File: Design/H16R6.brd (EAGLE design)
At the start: 30 x 34.6 mm, 113 parts, among them IC1 74LVC2T45HK3-7, P1 HEXABIT_17.32, U1 STM32G0B1CEU6N, X1 XTALL_CSTCE8M00G52

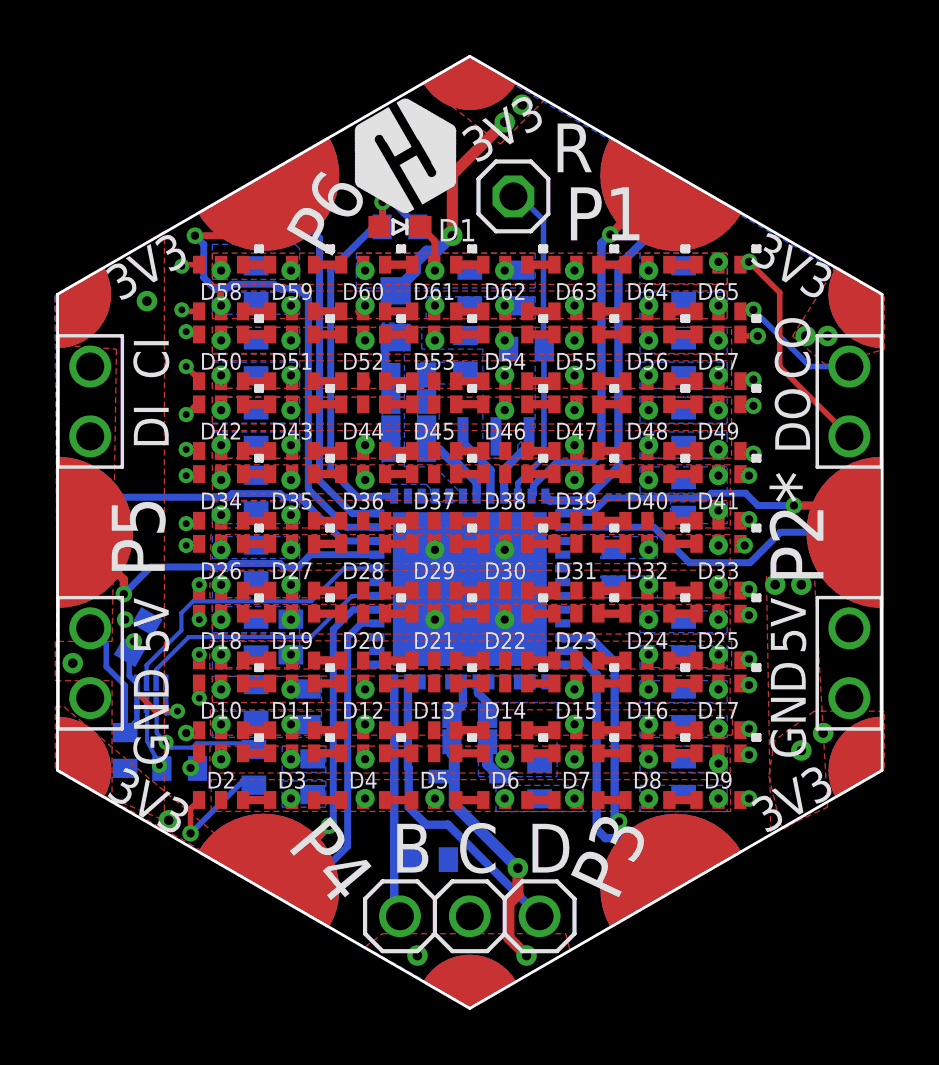
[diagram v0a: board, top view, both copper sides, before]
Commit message: no message
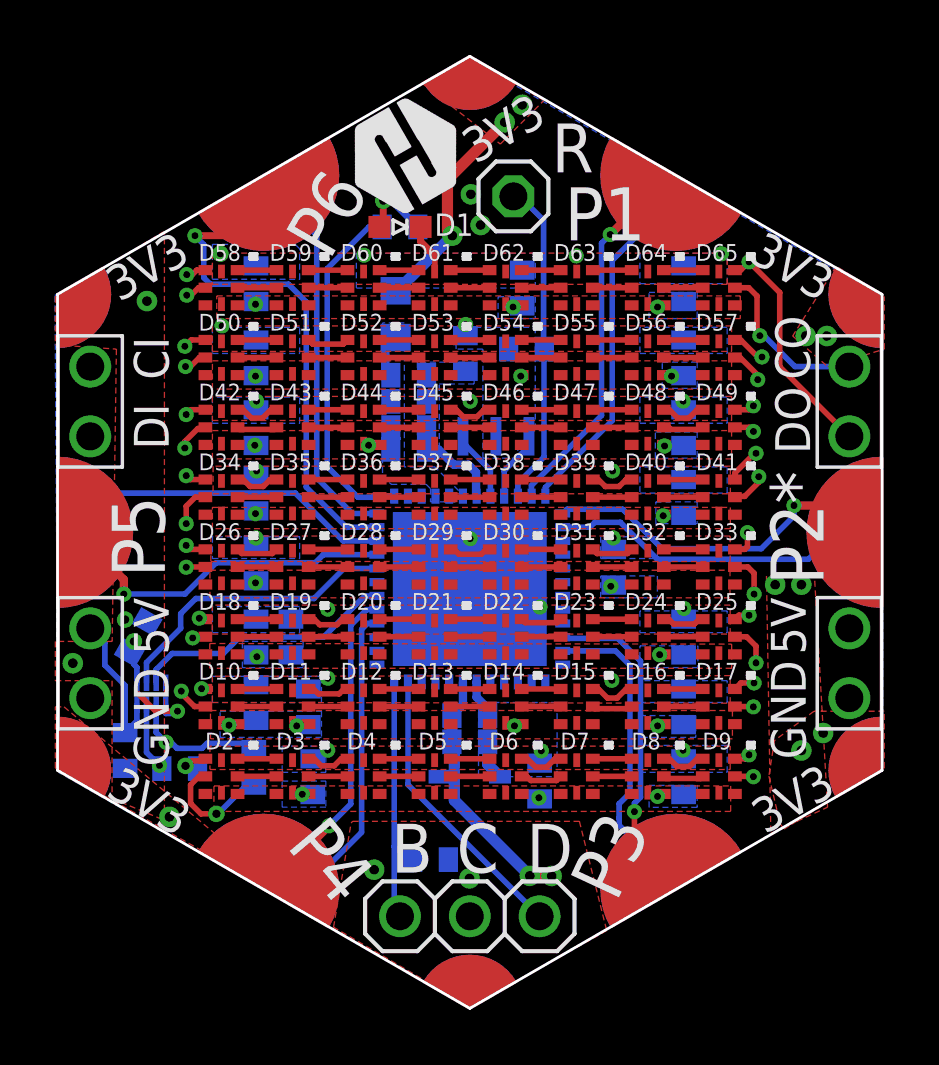
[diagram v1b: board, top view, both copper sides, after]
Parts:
- removed C1: 100nF, HEXABITZ_RCLS:C-0402
- moved SERIAL_IN 27.6 mm to (-13.8, 23.3)
- moved SERIAL_OUT 27.6 mm to (13.8, 23.3)
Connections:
- net +VS: now also D10.VDD1, D11.VDD1, D12.VDD1, D13.VDD1, D14.VDD1, D15.VDD1, D16.VDD1, D17.VDD1, D18.VDD1, D19.VDD1, D2.VDD1, D20.VDD1, D21.VDD1, D22.VDD1, D23.VDD1, D24.VDD1, D25.VDD1, D26.VDD1, D27.VDD1, D28.VDD1, D29.VDD1, D3.VDD1, D30.VDD1, D31.VDD1, D32.VDD1, D33.VDD1, D34.VDD1, D35.VDD1, D36.VDD1, D37.VDD1, D38.VDD1, D39.VDD1, D4.VDD1, D40.VDD1, D41.VDD1, D42.VDD1, D43.VDD1, D44.VDD1, D45.VDD1, D46.VDD1, D47.VDD1, D48.VDD1, D49.VDD1, D5.VDD1, D50.VDD1, D51.VDD1, D52.VDD1, D53.VDD1, D54.VDD1, D55.VDD1, D56.VDD1, D57.VDD1, D58.VDD1, D59.VDD1, D6.VDD1, D60.VDD1, D61.VDD1, D62.VDD1, D63.VDD1, D64.VDD1, D65.VDD1, D7.VDD1, D8.VDD1, D9.VDD1; no longer C1.1
- net CKI: now also SERIAL_IN.1; no longer SERIAL_OUT.1
- net CKO: now also D65.CO, SERIAL_OUT.1; no longer D65.CKO, SERIAL_IN.1
- net GND: no longer C1.2
- net L1_CLK: now also D10.CI, D9.CO; no longer D10.CKI, D9.CKO
- net L1_DATA: now also D10.DI, D9.DO; no longer D10.SDI, D9.SDO
- net L2_CLK: now also D17.CO, D18.CI; no longer D17.CKO, D18.CKI
- net L2_DATA: now also D17.DO, D18.DI; no longer D17.SDO, D18.SDI
- net L3_CLK: now also D25.CO, D26.CI; no longer D25.CKO, D26.CKI
- net L3_DATA: now also D25.DO, D26.DI; no longer D25.SDO, D26.SDI
- net L4_CLK: now also D33.CO, D34.CI; no longer D33.CKO, D34.CKI
- net L4_DATA: now also D33.DO, D34.DI; no longer D33.SDO, D34.SDI
- net L5_CLK: now also D41.CO, D42.CI; no longer D41.CKO, D42.CKI
- net L5_DATA: now also D41.DO, D42.DI; no longer D41.SDO, D42.SDI
- net L6_CLK: now also D49.CO, D50.CI; no longer D49.CKO, D50.CKI
- net L6_DATA: now also D49.DO, D50.DI; no longer D49.SDO, D50.SDI
- net L7_CLK: now also D57.CO, D58.CI; no longer D57.CKO, D58.CKI
- net L7_DATA: now also D57.DO, D58.DI; no longer D57.SDO, D58.SDI
- net N$1: now also D3.DO, D4.DI; no longer D3.SDO, D4.SDI
- net N$10: now also D8.CO, D9.CI; no longer D8.CKO, D9.CKI
- net N$100: now also D45.DO, D46.DI; no longer D45.SDO, D46.SDI
- net N$101: now also D45.CO, D46.CI; no longer D45.CKO, D46.CKI
- net N$102: now also D46.CO, D47.CI; no longer D46.CKO, D47.CKI
- net N$103: now also D46.DO, D47.DI; no longer D46.SDO, D47.SDI
- net N$104: now also D47.CO, D48.CI; no longer D47.CKO, D48.CKI
- net N$105: now also D47.DO, D48.DI; no longer D47.SDO, D48.SDI
- net N$106: now also D12.DO, D13.DI; no longer D12.SDO, D13.SDI
- net N$107: now also D13.DO, D14.DI; no longer D13.SDO, D14.SDI
- net N$108: now also D13.CO, D14.CI; no longer D13.CKO, D14.CKI
- net N$109: now also D14.CO, D15.CI; no longer D14.CKO, D15.CKI
- net N$11: now also D7.CO, D8.CI; no longer D7.CKO, D8.CKI
- net N$110: now also D14.DO, D15.DI; no longer D14.SDO, D15.SDI
- net N$111: now also D15.CO, D16.CI; no longer D15.CKO, D16.CKI
- net N$112: now also D15.DO, D16.DI; no longer D15.SDO, D16.SDI
- net N$113: now also D4.CO, D5.CI; no longer D4.CKO, D5.CKI
- net N$114: now also D4.DO, D5.DI; no longer D4.SDO, D5.SDI
- net N$115: now also D6.CO, D7.CI; no longer D6.CKO, D7.CKI
- net N$116: now also D6.DO, D7.DI; no longer D6.SDO, D7.SDI
- net N$119: now also D2.DI; no longer D2.SDI
- net N$12: now also D7.DO, D8.DI; no longer D7.SDO, D8.SDI
- net N$120: now also D2.CI; no longer D2.CKI
- net N$13: now also D5.CO, D6.CI; no longer D5.CKO, D6.CKI
- net N$14: now also D5.DO, D6.DI; no longer D5.SDO, D6.SDI
- net N$15: now also D16.CO, D17.CI; no longer D16.CKO, D17.CKI
- net N$16: now also D16.DO, D17.DI; no longer D16.SDO, D17.SDI
- net N$17: now also D10.CO, D11.CI; no longer D10.CKO, D11.CKI
- net N$18: now also D10.DO, D11.DI; no longer D10.SDO, D11.SDI
- net N$19: now also D11.CO, D12.CI; no longer D11.CKO, D12.CKI
- net N$2: now also D3.CO, D4.CI; no longer D3.CKO, D4.CKI
- net N$20: now also D11.DO, D12.DI; no longer D11.SDO, D12.SDI
- net N$21: now also D12.CO, D13.CI; no longer D12.CKO, D13.CKI
- net N$22: now also D18.CO, D19.CI; no longer D18.CKO, D19.CKI
- net N$23: now also D18.DO, D19.DI; no longer D18.SDO, D19.SDI
- net N$24: now also D19.CO, D20.CI; no longer D19.CKO, D20.CKI
- net N$25: now also D19.DO, D20.DI; no longer D19.SDO, D20.SDI
- net N$26: now also D20.CO, D21.CI; no longer D20.CKO, D21.CKI
- net N$27: now also D20.DO, D21.DI; no longer D20.SDO, D21.SDI
- net N$28: now also D21.CO, D22.CI; no longer D21.CKO, D22.CKI
- net N$29: now also D21.DO, D22.DI; no longer D21.SDO, D22.SDI
- net N$30: now also D22.CO, D23.CI; no longer D22.CKO, D23.CKI
- net N$31: now also D22.DO, D23.DI; no longer D22.SDO, D23.SDI
- net N$32: now also D23.CO, D24.CI; no longer D23.CKO, D24.CKI
- net N$33: now also D23.DO, D24.DI; no longer D23.SDO, D24.SDI
- net N$34: now also D24.CO, D25.CI; no longer D24.CKO, D25.CKI
- net N$35: now also D24.DO, D25.DI; no longer D24.SDO, D25.SDI
- net N$36: now also D26.CO, D27.CI; no longer D26.CKO, D27.CKI
- net N$37: now also D26.DO, D27.DI; no longer D26.SDO, D27.SDI
- net N$38: now also D27.CO, D28.CI; no longer D27.CKO, D28.CKI
- net N$39: now also D27.DO, D28.DI; no longer D27.SDO, D28.SDI
- net N$40: now also D28.CO, D29.CI; no longer D28.CKO, D29.CKI
- net N$41: now also D28.DO, D29.DI; no longer D28.SDO, D29.SDI
- net N$42: now also D29.CO, D30.CI; no longer D29.CKO, D30.CKI
- net N$43: now also D29.DO, D30.DI; no longer D29.SDO, D30.SDI
- net N$44: now also D31.CO, D32.CI; no longer D31.CKO, D32.CKI
- net N$45: now also D31.DO, D32.DI; no longer D31.SDO, D32.SDI
- net N$46: now also D30.CO, D31.CI; no longer D30.CKO, D31.CKI
- net N$47: now also D30.DO, D31.DI; no longer D30.SDO, D31.SDI
- net N$48: now also D32.CO, D33.CI; no longer D32.CKO, D33.CKI
- net N$49: now also D32.DO, D33.DI; no longer D32.SDO, D33.SDI
- net N$50: now also D34.CO, D35.CI; no longer D34.CKO, D35.CKI
- net N$51: now also D34.DO, D35.DI; no longer D34.SDO, D35.SDI
- net N$52: now also D35.CO, D36.CI; no longer D35.CKO, D36.CKI
- net N$53: now also D35.DO, D36.DI; no longer D35.SDO, D36.SDI
- net N$54: now also D36.CO, D37.CI; no longer D36.CKO, D37.CKI
- net N$55: now also D36.DO, D37.DI; no longer D36.SDO, D37.SDI
- net N$56: now also D37.CO, D38.CI; no longer D37.CKO, D38.CKI
- net N$57: now also D37.DO, D38.DI; no longer D37.SDO, D38.SDI
- net N$58: now also D38.CO, D39.CI; no longer D38.CKO, D39.CKI
- net N$59: now also D38.DO, D39.DI; no longer D38.SDO, D39.SDI
- net N$60: now also D40.CO, D41.CI; no longer D40.CKO, D41.CKI
- net N$61: now also D40.DO, D41.DI; no longer D40.SDO, D41.SDI
- net N$62: now also D39.CO, D40.CI; no longer D39.CKO, D40.CKI
- net N$63: now also D39.DO, D40.DI; no longer D39.SDO, D40.SDI
- net N$64: now also D48.CO, D49.CI; no longer D48.CKO, D49.CKI
- net N$65: now also D48.DO, D49.DI; no longer D48.SDO, D49.SDI
- net N$66: now also D56.CO, D57.CI; no longer D56.CKO, D57.CKI
- net N$67: now also D56.DO, D57.DI; no longer D56.SDO, D57.SDI
- net N$68: now also D64.CO, D65.CI; no longer D64.CKO, D65.CKI
- net N$69: now also D64.DO, D65.DI; no longer D64.SDO, D65.SDI
- net N$7: now also D2.DO, D3.DI; no longer D2.SDO, D3.SDI
- net N$70: now also D55.DO, D56.DI; no longer D55.SDO, D56.SDI
- net N$71: now also D55.CO, D56.CI; no longer D55.CKO, D56.CKI
- net N$72: now also D63.CO, D64.CI; no longer D63.CKO, D64.CKI
- net N$73: now also D63.DO, D64.DI; no longer D63.SDO, D64.SDI
- net N$74: now also D54.CO, D55.CI; no longer D54.CKO, D55.CKI
- net N$75: now also D54.DO, D55.DI; no longer D54.SDO, D55.SDI
- net N$76: now also D62.CO, D63.CI; no longer D62.CKO, D63.CKI
- net N$77: now also D62.DO, D63.DI; no longer D62.SDO, D63.SDI
- net N$78: now also D61.DO, D62.DI; no longer D61.SDO, D62.SDI
- net N$79: now also D61.CO, D62.CI; no longer D61.CKO, D62.CKI
- net N$8: now also D2.CO, D3.CI; no longer D2.CKO, D3.CKI
- net N$80: now also D60.CO, D61.CI; no longer D60.CKO, D61.CKI
- net N$81: now also D60.DO, D61.DI; no longer D60.SDO, D61.SDI
- net N$82: now also D59.CO, D60.CI; no longer D59.CKO, D60.CKI
- net N$83: now also D59.DO, D60.DI; no longer D59.SDO, D60.SDI
- net N$84: now also D58.DO, D59.DI; no longer D58.SDO, D59.SDI
- net N$85: now also D58.CO, D59.CI; no longer D58.CKO, D59.CKI
- net N$86: now also D53.DO, D54.DI; no longer D53.SDO, D54.SDI
- net N$87: now also D53.CO, D54.CI; no longer D53.CKO, D54.CKI
- net N$88: now also D51.CO, D52.CI; no longer D51.CKO, D52.CKI
- net N$89: now also D51.DO, D52.DI; no longer D51.SDO, D52.SDI
- net N$9: now also D8.DO, D9.DI; no longer D8.SDO, D9.SDI
- net N$90: now also D52.DO, D53.DI; no longer D52.SDO, D53.SDI
- net N$91: now also D52.CO, D53.CI; no longer D52.CKO, D53.CKI
- net N$92: now also D50.DO, D51.DI; no longer D50.SDO, D51.SDI
- net N$93: now also D50.CO, D51.CI; no longer D50.CKO, D51.CKI
- net N$94: now also D42.CO, D43.CI; no longer D42.CKO, D43.CKI
- net N$95: now also D42.DO, D43.DI; no longer D42.SDO, D43.SDI
- net N$96: now also D43.CO, D44.CI; no longer D43.CKO, D44.CKI
- net N$97: now also D43.DO, D44.DI; no longer D43.SDO, D44.SDI
- net N$98: now also D44.CO, D45.CI; no longer D44.CKO, D45.CKI
- net N$99: now also D44.DO, D45.DI; no longer D44.SDO, D45.SDI
- net SDI: now also SERIAL_IN.2; no longer SERIAL_OUT.2
- net SDO: now also D65.DO, SERIAL_OUT.2; no longer D65.SDO, SERIAL_IN.2
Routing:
- net L3_CLK: track 21.8 -> 24.4 mm
- net VDD: track 24.2 -> 21.9 mm
- net L1_CLK: track 22.5 -> 24.8 mm
- net L4_CLK: track 22.5 -> 24.7 mm
- net +VS: track 9.67 -> 11.8 mm, vias 44 -> 22
- net L5_CLK: track 22.6 -> 24.5 mm
- net L2_CLK: track 21.7 -> 23.0 mm
- net CKO: track 4.84 -> 6.14 mm
- net USART4_RX: track 14.0 -> 12.9 mm
- net USART2_TX: track 11.8 -> 12.9 mm
- net L1_DATA: track 21.7 -> 22.7 mm
- net L4_DATA: track 22.0 -> 23.0 mm
- net USART3_RX: track 10.4 -> 11.3 mm
- net USART3_TX: track 10.7 -> 11.5 mm
- net USART4_TX: track 14.1 -> 13.4 mm
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
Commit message: Replace the led APA-102-2020-6 with APA-102-2020-8
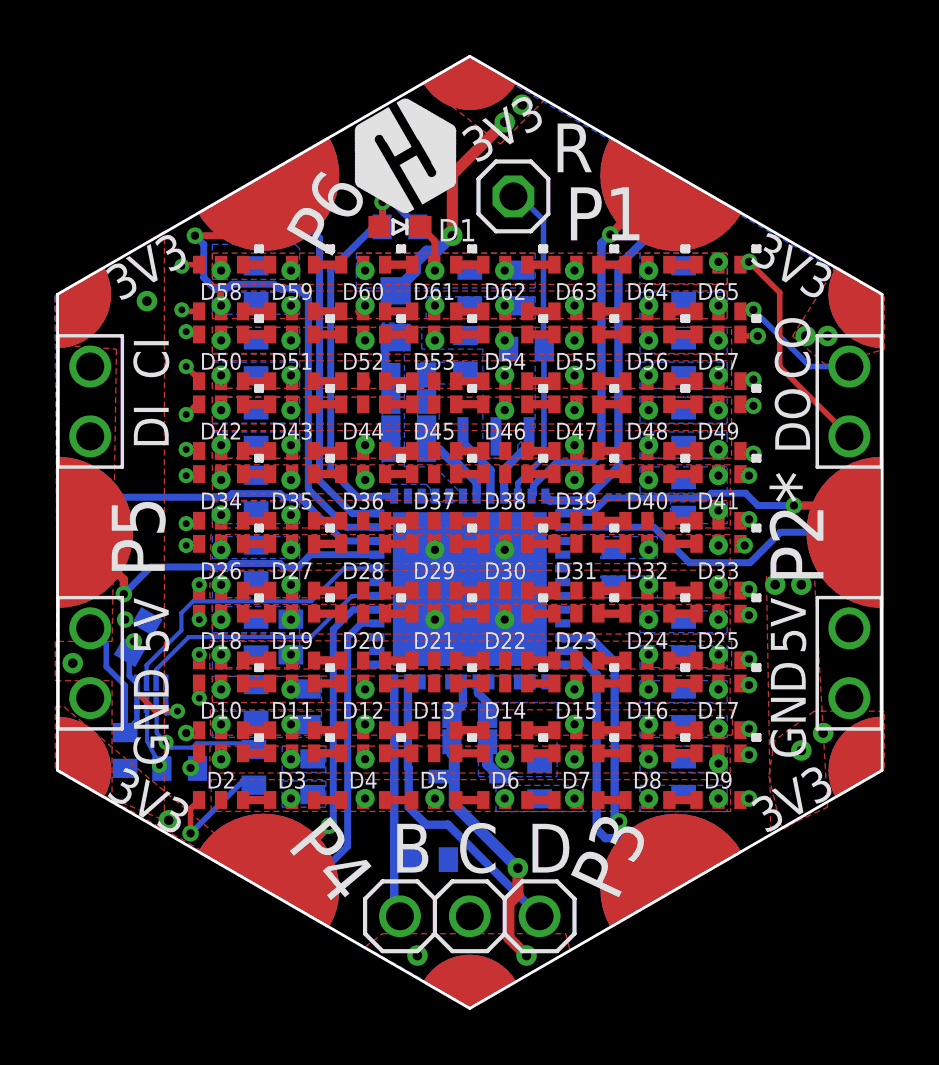
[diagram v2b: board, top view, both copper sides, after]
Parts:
- added C1: 100nF, HEXABITZ_RCLS:C-0402
- moved SERIAL_IN 27.6 mm to (13.8, 23.3)
- moved SERIAL_OUT 27.6 mm to (-13.8, 23.3)
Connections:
- net +VS: now also C1.1; no longer D10.VDD1, D11.VDD1, D12.VDD1, D13.VDD1, D14.VDD1, D15.VDD1, D16.VDD1, D17.VDD1, D18.VDD1, D19.VDD1, D2.VDD1, D20.VDD1, D21.VDD1, D22.VDD1, D23.VDD1, D24.VDD1, D25.VDD1, D26.VDD1, D27.VDD1, D28.VDD1, D29.VDD1, D3.VDD1, D30.VDD1, D31.VDD1, D32.VDD1, D33.VDD1, D34.VDD1, D35.VDD1, D36.VDD1, D37.VDD1, D38.VDD1, D39.VDD1, D4.VDD1, D40.VDD1, D41.VDD1, D42.VDD1, D43.VDD1, D44.VDD1, D45.VDD1, D46.VDD1, D47.VDD1, D48.VDD1, D49.VDD1, D5.VDD1, D50.VDD1, D51.VDD1, D52.VDD1, D53.VDD1, D54.VDD1, D55.VDD1, D56.VDD1, D57.VDD1, D58.VDD1, D59.VDD1, D6.VDD1, D60.VDD1, D61.VDD1, D62.VDD1, D63.VDD1, D64.VDD1, D65.VDD1, D7.VDD1, D8.VDD1, D9.VDD1
- net CKI: now also SERIAL_OUT.1; no longer SERIAL_IN.1
- net CKO: now also D65.CKO, SERIAL_IN.1; no longer D65.CO, SERIAL_OUT.1
- net GND: now also C1.2
- net L1_CLK: now also D10.CKI, D9.CKO; no longer D10.CI, D9.CO
- net L1_DATA: now also D10.SDI, D9.SDO; no longer D10.DI, D9.DO
- net L2_CLK: now also D17.CKO, D18.CKI; no longer D17.CO, D18.CI
- net L2_DATA: now also D17.SDO, D18.SDI; no longer D17.DO, D18.DI
- net L3_CLK: now also D25.CKO, D26.CKI; no longer D25.CO, D26.CI
- net L3_DATA: now also D25.SDO, D26.SDI; no longer D25.DO, D26.DI
- net L4_CLK: now also D33.CKO, D34.CKI; no longer D33.CO, D34.CI
- net L4_DATA: now also D33.SDO, D34.SDI; no longer D33.DO, D34.DI
- net L5_CLK: now also D41.CKO, D42.CKI; no longer D41.CO, D42.CI
- net L5_DATA: now also D41.SDO, D42.SDI; no longer D41.DO, D42.DI
- net L6_CLK: now also D49.CKO, D50.CKI; no longer D49.CO, D50.CI
- net L6_DATA: now also D49.SDO, D50.SDI; no longer D49.DO, D50.DI
- net L7_CLK: now also D57.CKO, D58.CKI; no longer D57.CO, D58.CI
- net L7_DATA: now also D57.SDO, D58.SDI; no longer D57.DO, D58.DI
- net N$1: now also D3.SDO, D4.SDI; no longer D3.DO, D4.DI
- net N$10: now also D8.CKO, D9.CKI; no longer D8.CO, D9.CI
- net N$100: now also D45.SDO, D46.SDI; no longer D45.DO, D46.DI
- net N$101: now also D45.CKO, D46.CKI; no longer D45.CO, D46.CI
- net N$102: now also D46.CKO, D47.CKI; no longer D46.CO, D47.CI
- net N$103: now also D46.SDO, D47.SDI; no longer D46.DO, D47.DI
- net N$104: now also D47.CKO, D48.CKI; no longer D47.CO, D48.CI
- net N$105: now also D47.SDO, D48.SDI; no longer D47.DO, D48.DI
- net N$106: now also D12.SDO, D13.SDI; no longer D12.DO, D13.DI
- net N$107: now also D13.SDO, D14.SDI; no longer D13.DO, D14.DI
- net N$108: now also D13.CKO, D14.CKI; no longer D13.CO, D14.CI
- net N$109: now also D14.CKO, D15.CKI; no longer D14.CO, D15.CI
- net N$11: now also D7.CKO, D8.CKI; no longer D7.CO, D8.CI
- net N$110: now also D14.SDO, D15.SDI; no longer D14.DO, D15.DI
- net N$111: now also D15.CKO, D16.CKI; no longer D15.CO, D16.CI
- net N$112: now also D15.SDO, D16.SDI; no longer D15.DO, D16.DI
- net N$113: now also D4.CKO, D5.CKI; no longer D4.CO, D5.CI
- net N$114: now also D4.SDO, D5.SDI; no longer D4.DO, D5.DI
- net N$115: now also D6.CKO, D7.CKI; no longer D6.CO, D7.CI
- net N$116: now also D6.SDO, D7.SDI; no longer D6.DO, D7.DI
- net N$119: now also D2.SDI; no longer D2.DI
- net N$12: now also D7.SDO, D8.SDI; no longer D7.DO, D8.DI
- net N$120: now also D2.CKI; no longer D2.CI
- net N$13: now also D5.CKO, D6.CKI; no longer D5.CO, D6.CI
- net N$14: now also D5.SDO, D6.SDI; no longer D5.DO, D6.DI
- net N$15: now also D16.CKO, D17.CKI; no longer D16.CO, D17.CI
- net N$16: now also D16.SDO, D17.SDI; no longer D16.DO, D17.DI
- net N$17: now also D10.CKO, D11.CKI; no longer D10.CO, D11.CI
- net N$18: now also D10.SDO, D11.SDI; no longer D10.DO, D11.DI
- net N$19: now also D11.CKO, D12.CKI; no longer D11.CO, D12.CI
- net N$2: now also D3.CKO, D4.CKI; no longer D3.CO, D4.CI
- net N$20: now also D11.SDO, D12.SDI; no longer D11.DO, D12.DI
- net N$21: now also D12.CKO, D13.CKI; no longer D12.CO, D13.CI
- net N$22: now also D18.CKO, D19.CKI; no longer D18.CO, D19.CI
- net N$23: now also D18.SDO, D19.SDI; no longer D18.DO, D19.DI
- net N$24: now also D19.CKO, D20.CKI; no longer D19.CO, D20.CI
- net N$25: now also D19.SDO, D20.SDI; no longer D19.DO, D20.DI
- net N$26: now also D20.CKO, D21.CKI; no longer D20.CO, D21.CI
- net N$27: now also D20.SDO, D21.SDI; no longer D20.DO, D21.DI
- net N$28: now also D21.CKO, D22.CKI; no longer D21.CO, D22.CI
- net N$29: now also D21.SDO, D22.SDI; no longer D21.DO, D22.DI
- net N$30: now also D22.CKO, D23.CKI; no longer D22.CO, D23.CI
- net N$31: now also D22.SDO, D23.SDI; no longer D22.DO, D23.DI
- net N$32: now also D23.CKO, D24.CKI; no longer D23.CO, D24.CI
- net N$33: now also D23.SDO, D24.SDI; no longer D23.DO, D24.DI
- net N$34: now also D24.CKO, D25.CKI; no longer D24.CO, D25.CI
- net N$35: now also D24.SDO, D25.SDI; no longer D24.DO, D25.DI
- net N$36: now also D26.CKO, D27.CKI; no longer D26.CO, D27.CI
- net N$37: now also D26.SDO, D27.SDI; no longer D26.DO, D27.DI
- net N$38: now also D27.CKO, D28.CKI; no longer D27.CO, D28.CI
- net N$39: now also D27.SDO, D28.SDI; no longer D27.DO, D28.DI
- net N$40: now also D28.CKO, D29.CKI; no longer D28.CO, D29.CI
- net N$41: now also D28.SDO, D29.SDI; no longer D28.DO, D29.DI
- net N$42: now also D29.CKO, D30.CKI; no longer D29.CO, D30.CI
- net N$43: now also D29.SDO, D30.SDI; no longer D29.DO, D30.DI
- net N$44: now also D31.CKO, D32.CKI; no longer D31.CO, D32.CI
- net N$45: now also D31.SDO, D32.SDI; no longer D31.DO, D32.DI
- net N$46: now also D30.CKO, D31.CKI; no longer D30.CO, D31.CI
- net N$47: now also D30.SDO, D31.SDI; no longer D30.DO, D31.DI
- net N$48: now also D32.CKO, D33.CKI; no longer D32.CO, D33.CI
- net N$49: now also D32.SDO, D33.SDI; no longer D32.DO, D33.DI
- net N$50: now also D34.CKO, D35.CKI; no longer D34.CO, D35.CI
- net N$51: now also D34.SDO, D35.SDI; no longer D34.DO, D35.DI
- net N$52: now also D35.CKO, D36.CKI; no longer D35.CO, D36.CI
- net N$53: now also D35.SDO, D36.SDI; no longer D35.DO, D36.DI
- net N$54: now also D36.CKO, D37.CKI; no longer D36.CO, D37.CI
- net N$55: now also D36.SDO, D37.SDI; no longer D36.DO, D37.DI
- net N$56: now also D37.CKO, D38.CKI; no longer D37.CO, D38.CI
- net N$57: now also D37.SDO, D38.SDI; no longer D37.DO, D38.DI
- net N$58: now also D38.CKO, D39.CKI; no longer D38.CO, D39.CI
- net N$59: now also D38.SDO, D39.SDI; no longer D38.DO, D39.DI
- net N$60: now also D40.CKO, D41.CKI; no longer D40.CO, D41.CI
- net N$61: now also D40.SDO, D41.SDI; no longer D40.DO, D41.DI
- net N$62: now also D39.CKO, D40.CKI; no longer D39.CO, D40.CI
- net N$63: now also D39.SDO, D40.SDI; no longer D39.DO, D40.DI
- net N$64: now also D48.CKO, D49.CKI; no longer D48.CO, D49.CI
- net N$65: now also D48.SDO, D49.SDI; no longer D48.DO, D49.DI
- net N$66: now also D56.CKO, D57.CKI; no longer D56.CO, D57.CI
- net N$67: now also D56.SDO, D57.SDI; no longer D56.DO, D57.DI
- net N$68: now also D64.CKO, D65.CKI; no longer D64.CO, D65.CI
- net N$69: now also D64.SDO, D65.SDI; no longer D64.DO, D65.DI
- net N$7: now also D2.SDO, D3.SDI; no longer D2.DO, D3.DI
- net N$70: now also D55.SDO, D56.SDI; no longer D55.DO, D56.DI
- net N$71: now also D55.CKO, D56.CKI; no longer D55.CO, D56.CI
- net N$72: now also D63.CKO, D64.CKI; no longer D63.CO, D64.CI
- net N$73: now also D63.SDO, D64.SDI; no longer D63.DO, D64.DI
- net N$74: now also D54.CKO, D55.CKI; no longer D54.CO, D55.CI
- net N$75: now also D54.SDO, D55.SDI; no longer D54.DO, D55.DI
- net N$76: now also D62.CKO, D63.CKI; no longer D62.CO, D63.CI
- net N$77: now also D62.SDO, D63.SDI; no longer D62.DO, D63.DI
- net N$78: now also D61.SDO, D62.SDI; no longer D61.DO, D62.DI
- net N$79: now also D61.CKO, D62.CKI; no longer D61.CO, D62.CI
- net N$8: now also D2.CKO, D3.CKI; no longer D2.CO, D3.CI
- net N$80: now also D60.CKO, D61.CKI; no longer D60.CO, D61.CI
- net N$81: now also D60.SDO, D61.SDI; no longer D60.DO, D61.DI
- net N$82: now also D59.CKO, D60.CKI; no longer D59.CO, D60.CI
- net N$83: now also D59.SDO, D60.SDI; no longer D59.DO, D60.DI
- net N$84: now also D58.SDO, D59.SDI; no longer D58.DO, D59.DI
- net N$85: now also D58.CKO, D59.CKI; no longer D58.CO, D59.CI
- net N$86: now also D53.SDO, D54.SDI; no longer D53.DO, D54.DI
- net N$87: now also D53.CKO, D54.CKI; no longer D53.CO, D54.CI
- net N$88: now also D51.CKO, D52.CKI; no longer D51.CO, D52.CI
- net N$89: now also D51.SDO, D52.SDI; no longer D51.DO, D52.DI
- net N$9: now also D8.SDO, D9.SDI; no longer D8.DO, D9.DI
- net N$90: now also D52.SDO, D53.SDI; no longer D52.DO, D53.DI
- net N$91: now also D52.CKO, D53.CKI; no longer D52.CO, D53.CI
- net N$92: now also D50.SDO, D51.SDI; no longer D50.DO, D51.DI
- net N$93: now also D50.CKO, D51.CKI; no longer D50.CO, D51.CI
- net N$94: now also D42.CKO, D43.CKI; no longer D42.CO, D43.CI
- net N$95: now also D42.SDO, D43.SDI; no longer D42.DO, D43.DI
- net N$96: now also D43.CKO, D44.CKI; no longer D43.CO, D44.CI
- net N$97: now also D43.SDO, D44.SDI; no longer D43.DO, D44.DI
- net N$98: now also D44.CKO, D45.CKI; no longer D44.CO, D45.CI
- net N$99: now also D44.SDO, D45.SDI; no longer D44.DO, D45.DI
- net SDI: now also SERIAL_OUT.2; no longer SERIAL_IN.2
- net SDO: now also D65.SDO, SERIAL_IN.2; no longer D65.DO, SERIAL_OUT.2
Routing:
- net L3_CLK: track 24.4 -> 21.8 mm
- net VDD: track 21.9 -> 24.2 mm
- net L1_CLK: track 24.8 -> 22.5 mm
- net L4_CLK: track 24.7 -> 22.5 mm
- net +VS: track 11.8 -> 9.67 mm, vias 22 -> 44
- net L5_CLK: track 24.5 -> 22.6 mm
- net L2_CLK: track 23.0 -> 21.7 mm
- net CKO: track 6.14 -> 4.84 mm
- net USART4_RX: track 12.9 -> 14.0 mm
- net USART2_TX: track 12.9 -> 11.8 mm
- net L1_DATA: track 22.7 -> 21.7 mm
- net L4_DATA: track 23.0 -> 22.0 mm
- net USART3_RX: track 11.3 -> 10.4 mm
- net USART3_TX: track 11.5 -> 10.7 mm
- net USART4_TX: track 13.4 -> 14.1 mm
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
